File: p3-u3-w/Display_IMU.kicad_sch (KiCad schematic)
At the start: 18 parts, among them J2 Display, J5 UART, SW1 SW_SPST, SW3 SW_SPST, SW4 SW_SPST, SW5 SW_SPST, SW6 SW_SPST, SW7 SW_SPST, U1 LSM6DSM

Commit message: changed some routing
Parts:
- C13, C14: footprint Capacitor_SMD:C_0603_1608Metric -> Capacitor_SMD:C_0402_1005Metric
- R1, R17, R18, R19, R2, R20, R21: footprint Resistor_SMD:R_0603_1608Metric -> Resistor_SMD:R_0402_1005Metric
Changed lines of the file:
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@@
 			)
 		)
-		(property "Footprint" "Resistor_SMD:R_0603_1608Metric"
+		(property "Footprint" "Resistor_SMD:R_0402_1005Metric"
 			(at 63.5 115.062 90)
 			(effects
@@
 			)
 		)
-		(property "Footprint" "Capacitor_SMD:C_0603_1608Metric"
+		(property "Footprint" "Capacitor_SMD:C_0402_1005Metric"
 			(at 167.3352 63.5 0)
 			(effects
@@
 			)
 		)
-		(property "Footprint" "Resistor_SMD:R_0603_1608Metric"
+		(property "Footprint" "Resistor_SMD:R_0402_1005Metric"
 			(at 63.5 174.752 90)
 			(effects
@@
 			)
 		)
-		(property "Footprint" "Resistor_SMD:R_0603_1608Metric"
+		(property "Footprint" "Resistor_SMD:R_0402_1005Metric"
 			(at 63.5 129.032 90)
 			(effects
@@
 			)
 		)
-		(property "Footprint" "Resistor_SMD:R_0603_1608Metric"
+		(property "Footprint" "Resistor_SMD:R_0402_1005Metric"
 			(at 63.5 101.092 90)
 			(effects
@@
 			)
 		)
-		(property "Footprint" "Resistor_SMD:R_0603_1608Metric"
+		(property "Footprint" "Resistor_SMD:R_0402_1005Metric"
 			(at 123.952 35.56 90)
 			(effects
@@
 			)
 		)
-		(property "Footprint" "Resistor_SMD:R_0603_1608Metric"
+		(property "Footprint" "Resistor_SMD:R_0402_1005Metric"
 			(at 63.5 159.512 90)
 			(effects
@@
 			)
 		)
-		(property "Footprint" "Capacitor_SMD:C_0603_1608Metric"
+		(property "Footprint" "Capacitor_SMD:C_0402_1005Metric"
 			(at 157.1752 63.5 0)
 			(effects
@@
 			)
 		)
-		(property "Footprint" "Resistor_SMD:R_0603_1608Metric"
+		(property "Footprint" "Resistor_SMD:R_0402_1005Metric"
 			(at 63.5 144.272 90)
 			(effects

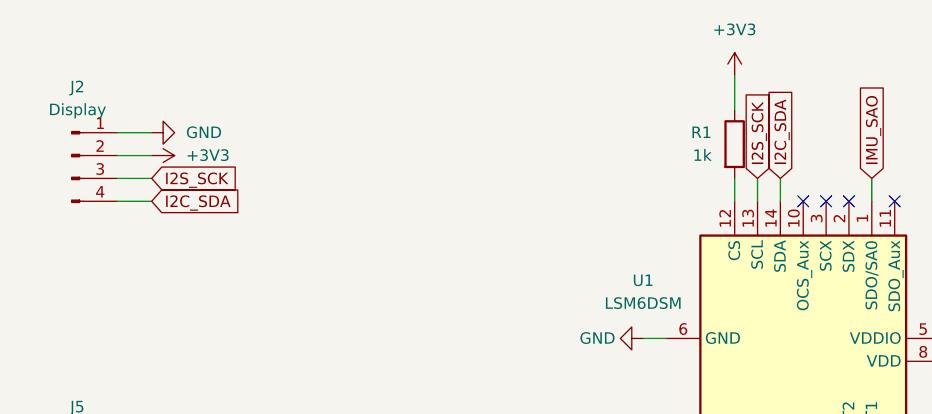
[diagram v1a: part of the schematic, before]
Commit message: added in some more routing.
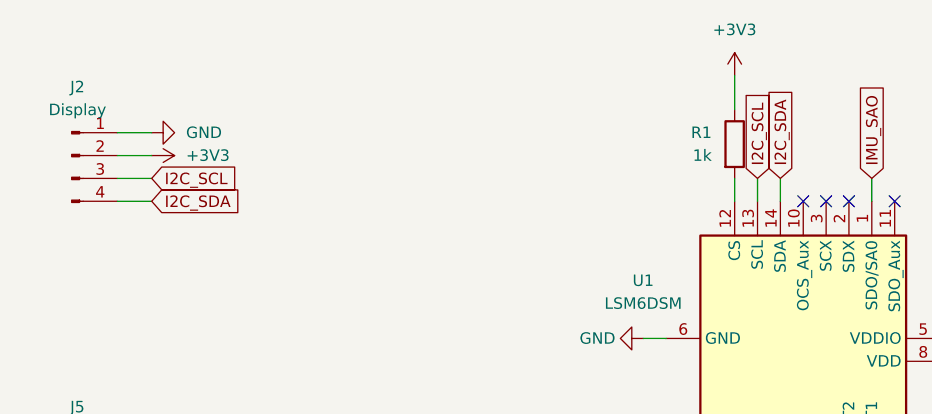
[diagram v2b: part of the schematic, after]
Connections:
- net I2S_SCK renamed I2C_SCL
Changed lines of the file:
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@@
+		)
+	)
+	(global_label "I2C_SCL"
+		(shape input)
+		(at 128.27 39.37 90)
+		(fields_autoplaced yes)
+		(effects
+			(font
+				(size 1.27 1.27)
+			)
+			(justify left)
+		)
+		(property "Intersheetrefs" "${INTERSHEET_REFS}"
+			(at 128.27 28.8253 90)
+			(effects
+				(font
+					(size 1.27 1.27)
+				)
+				(justify left)
+				(hide yes)
+			)
 		)
 	)
@@
 		)
 	)
+	(global_label "I2C_SCL"
+		(shape input)
+		(at 60.96 39.37 0)
+		(fields_autoplaced yes)
+		(effects
+			(font
+				(size 1.27 1.27)
+			)
+			(justify left)
+		)
+		(property "Intersheetrefs" "${INTERSHEET_REFS}"
+			(at 71.5047 39.37 0)
+			(effects
+				(font
+					(size 1.27 1.27)
+				)
+				(justify left)
+				(hide yes)
+			)
+		)
+	)
 	(global_label "BTN_VOL+"
 		(shape input)
@@
 		)
 	)
-	(global_label "I2S_SCK"
-		(shape input)
-		(at 128.27 39.37 90)
-		(fields_autoplaced yes)
-		(effects
-			(font
-				(size 1.27 1.27)
-			)
-			(justify left)
-		)
-		(property "Intersheetrefs" "${INTERSHEET_REFS}"
-			(at 128.27 28.6439 90)
-			(effects
-				(font
-					(size 1.27 1.27)
-				)
-				(justify left)
-				(hide yes)
-			)
-		)
-	)
 	(global_label "IMU_SAO"
 		(shape input)
@@
 			(effects
 				(font
-					(size 1.27 1.27)
-				)
-				(justify left)
-				(hide yes)
-			)
-		)
-	)
-	(global_label "I2S_SCK"
-		(shape input)
-		(at 60.96 39.37 0)
-		(fields_autoplaced yes)
-		(effects
-			(font
-				(size 1.27 1.27)
-			)
-			(justify left)
-		)
-		(property "Intersheetrefs" "${INTERSHEET_REFS}"
-			(at 71.6861 39.37 0)
-			(effects
-				(font
